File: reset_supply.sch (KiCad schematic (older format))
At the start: 32 parts, among them Q201 CSD18543Q3A, U201 LM25088MH-1

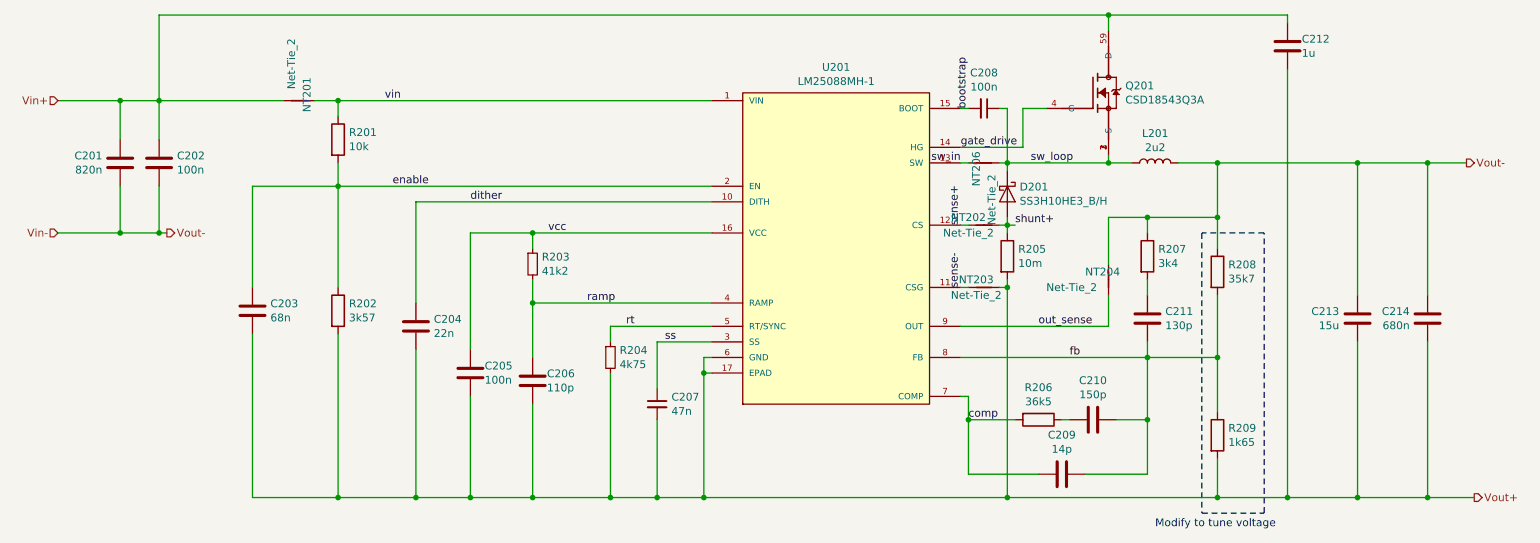
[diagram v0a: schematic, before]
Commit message: spun up integrated version
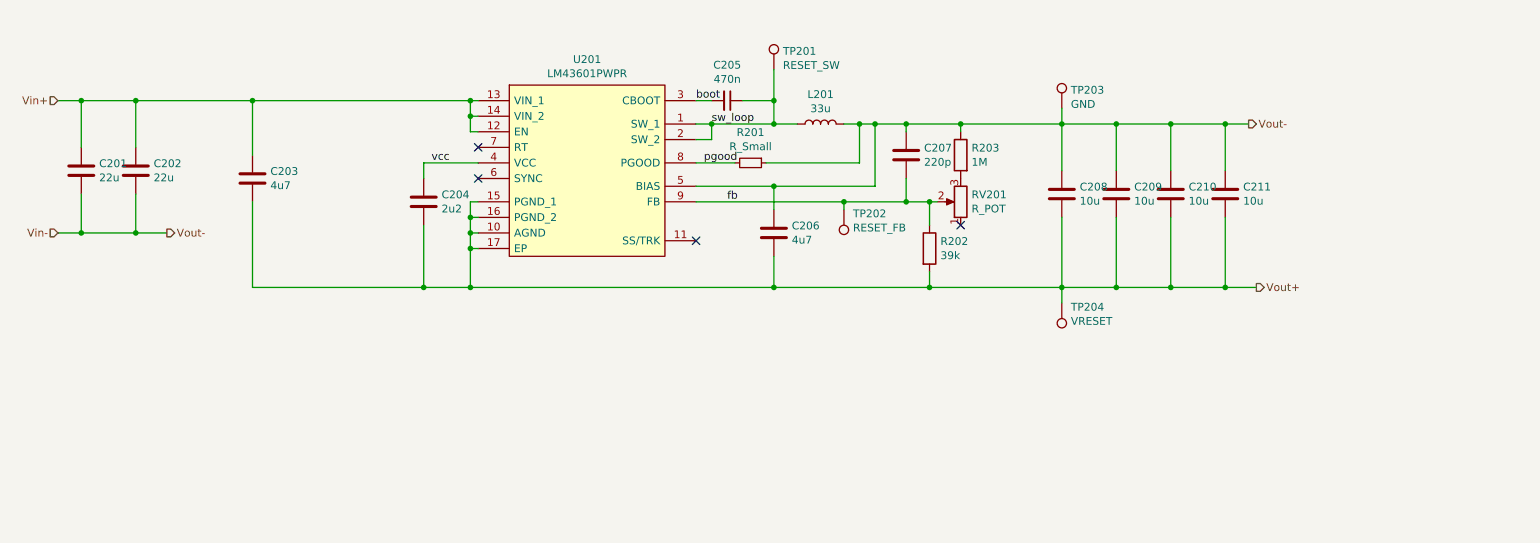
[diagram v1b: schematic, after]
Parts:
- removed C205: 100n, Capacitors_SMD:C_0805_HandSoldering, symbol device:C
- removed C207: 47n, Capacitors_SMD:C_0805_HandSoldering, symbol device:C_Small
- removed C208: 100n, Capacitors_SMD:C_0805_HandSoldering, symbol device:C_Small
- removed C212: 1u, Capacitors_SMD:C_0805_HandSoldering, symbol device:C
- removed C213: 15u, Capacitors_SMD:C_2220_HandSoldering, symbol device:C
- removed C214: 680n, Capacitors_SMD:C_0805_HandSoldering, symbol device:C
- removed D201: SS3H10HE3_B/H, Diodes_SMD:D_SMC, symbol device:D_Schottky
- removed NT201, NT204, NT206: Net-Tie_2, Oddities:NetTie-I_SMD, symbol device:Net-Tie_2
- removed NT202, NT203: Net-Tie_2, net_ties:NET-TIE-0.3mm, symbol device:Net-Tie_2
- removed Q201: CSD18543Q3A, SON65P300X315X90-9N, symbol CSD18543Q3A:CSD18543Q3A
- removed R201: 10k, Resistors_SMD:R_0805_HandSoldering, symbol device:R
- removed R203: 41k2, Resistors_SMD:R_0805_HandSoldering, symbol device:R_Small
- removed R204: 4k75, Resistors_SMD:R_0805_HandSoldering, symbol device:R_Small
- removed R205: 10m, Resistors_SMD:R_0612, symbol device:R
- removed R206: 36k5, Resistors_SMD:R_0805_HandSoldering, symbol device:R
- removed R207: 3k4, Resistors_SMD:R_0805_HandSoldering, symbol device:R
- removed R208: 35k7, Resistors_SMD:R_0805_HandSoldering, symbol device:R
- removed R209: 1k65, Resistors_SMD:R_0805_HandSoldering, symbol device:R
- removed U201: LM25088MH-1, LM25088MH-1:SOP65P640X110-17N, symbol d4100_mod_board_full-rescue:LM25088MH-1-LM25088MH-1
- added C205: 470n, Capacitors_SMD:C_0805_HandSoldering, symbol device:C_Small
- added C207: 220p, Capacitors_SMD:C_0805_HandSoldering, symbol device:C
- added C208: 10u, Capacitors_SMD:C_1210_HandSoldering, symbol device:C
- added R201: R_Small, Resistors_SMD:R_0805_HandSoldering, symbol device:R_Small
- added R203: 1M, Resistors_SMD:R_0805_HandSoldering, symbol device:R
- added RV201: R_POT, SamacSys_Parts:PVG5A502C03R00, symbol device:R_POT
- added TP201: RESET_SW, Measurement_Points:Measurement_Point_Round-TH_Small, symbol conn:TEST_1P
- added TP202: RESET_FB, Measurement_Points:Measurement_Point_Round-TH_Small, symbol conn:TEST_1P
- added TP203: GND, Measurement_Points:Measurement_Point_Square-TH_Small, symbol conn:TEST_1P
- added TP204: VRESET, Measurement_Points:Measurement_Point_Round-TH_Small, symbol conn:TEST_1P
- added U201: LM43601PWPR, SamacSys_Parts:SOP65P640X120-17N, symbol SamacSys_Parts:LM43601PWPR
- C201: value 820n -> 22u; footprint Capacitors_SMD:C_0805_HandSoldering -> Capacitors_SMD:C_1210_HandSoldering; Vendor (none) -> https://www.mouser.com/ProductDetail/Murata/GRM32ER61C226ME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
- C202: value 100n -> 22u; footprint Capacitors_SMD:C_0805_HandSoldering -> Capacitors_SMD:C_1210_HandSoldering; Vendor https://www.mouser.com/ProductDetail/Taiyo-Yuden/TMK212BJ47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 -> https://www.mouser.com/ProductDetail/Murata/GRM32ER61C226ME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
- C203: value 68n -> 4u7; Vendor https://www.mouser.com/ProductDetail/KEMET/C0805C683K5RACAU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 -> https://www.mouser.com/ProductDetail/Murata-Electronics/GRM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
- C204: value 22n -> 2u2; Vendor https://www.mouser.com/ProductDetail/KEMET/C0805C223K5RACTU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 -> https://www.mouser.com/ProductDetail/Taiyo-Yuden/EMK212BJ22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
- C206: value 110p -> 4u7; Vendor (none) -> https://www.mouser.com/ProductDetail/Taiyo-Yuden/TMK212BJ47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
- C209: value 14p -> 10u; footprint Capacitors_SMD:C_0805_HandSoldering -> Capacitors_SMD:C_1210_HandSoldering; Vendor (none) -> https://www.mouser.com/ProductDetail/Murata-Electronics/GRM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
- C210: value 150p -> 10u; footprint Capacitors_SMD:C_0805_HandSoldering -> Capacitors_SMD:C_1210_HandSoldering; Vendor (none) -> https://www.mouser.com/ProductDetail/Murata-Electronics/GRM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
- C211: value 130p -> 10u; footprint Capacitors_SMD:C_0805_HandSoldering -> Capacitors_SMD:C_1210_HandSoldering; Vendor (none) -> https://www.mouser.com/ProductDetail/Murata-Electronics/GRM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
- L201: value 2u2 -> 33u; footprint d4100_mod_board:WE-LHMI_7030 -> SamacSys_Parts:SRN4012TA; Vendor https://www.mouser.com/ProductDetail/Wurth-Elektronik/74437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 -> https://www.mouser.com/ProductDetail/Bourns/SRN3015-330M?qs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
- R202: value 3k57 -> 39k; Vendor https://www.mouser.com/ProductDetail/Panasonic/ERJ-6ENF3571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 -> https://www.mouser.com/ProductDetail/Vishay-Dale/CRCW080539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
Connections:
- net comp is gone; now on net Vout+: C209.2
- net dither is gone; now on net vcc: C204.1
- net ramp is gone; now on net Vin-: C206.1
- net Vin+: now also C203.1, U201.12 (EN), U201.13 (VIN_1), U201.14 (VIN_2)
- net Vin-: now also C209.1, C210.1, C211.1, C207.1, C208.1, R201.1, R203.1, TP203.1, U201.5 (BIAS)
- net Vout+: now also C210.2, C211.2, C208.2, TP204.1, U201.10 (AGND), U201.15 (PGND_1), U201.16 (PGND_2), U201.17 (EP)
- net fb: now also R202.1, C207.2, RV201.2, TP202.1, U201.9 (FB); no longer C209.1, C210.1, C211.1
- net sw_loop: now also C205.1, TP201.1, U201.1 (SW_1), U201.2 (SW_2)
- net vcc: now also U201.4 (VCC)
- removed net enable: C203.1, R202.1
- new net: R203.2, RV201.3
- new net boot: C205.2, U201.3 (CBOOT)
- new net pgood: R201.2, U201.8 (PGOOD)
- no-connect marks 0 -> 4
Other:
- note removed: "Modify to tune voltage"
